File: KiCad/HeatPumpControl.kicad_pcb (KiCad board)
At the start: 2 copper layers, 38.2 x 37.4 mm, 45 parts, among them J1 Conn_01x04_Male, J2 Conn_01x04_Male, J3 Conn_01x04_Male, J4 Conn_01x03_Male, Q1 2N2222A, Q2 Q_PMOS_GDS, U3 XIAO-ESP32-C6-SMD

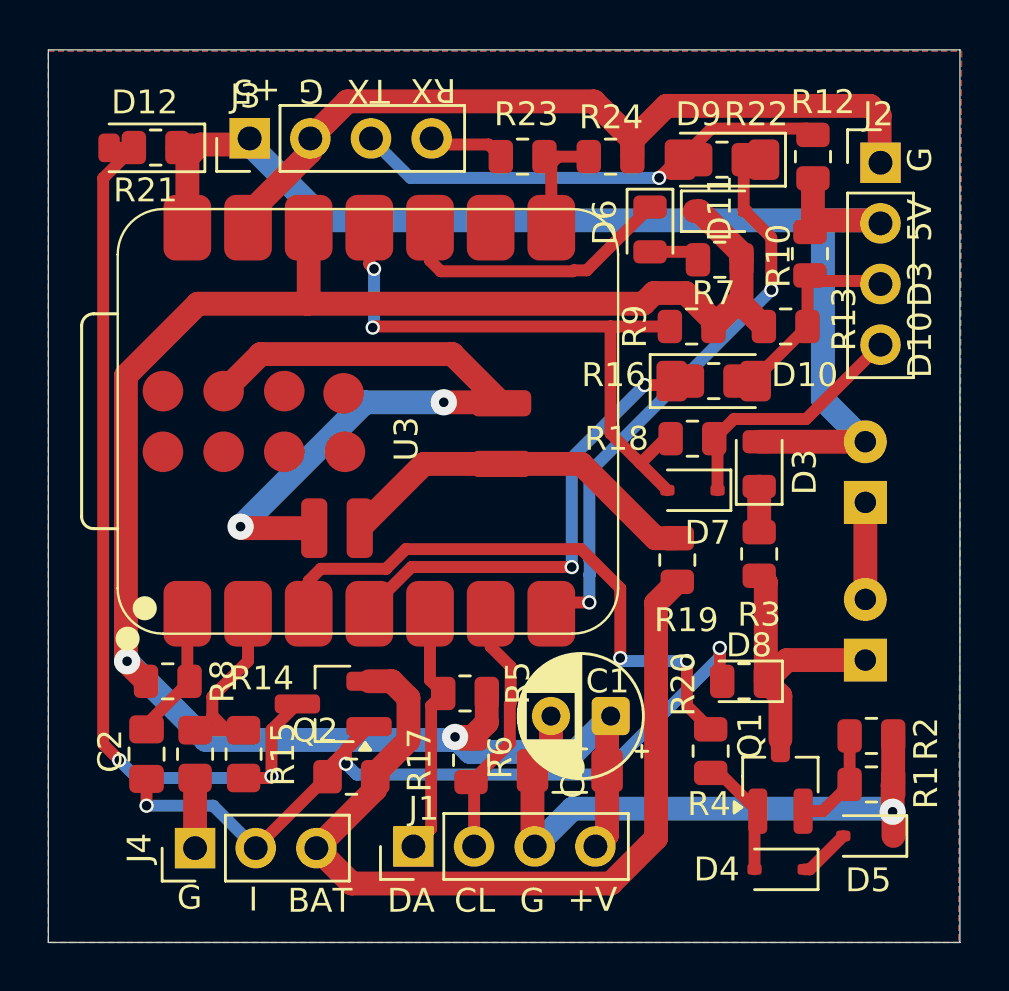
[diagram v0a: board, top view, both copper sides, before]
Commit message: Fill zones updated
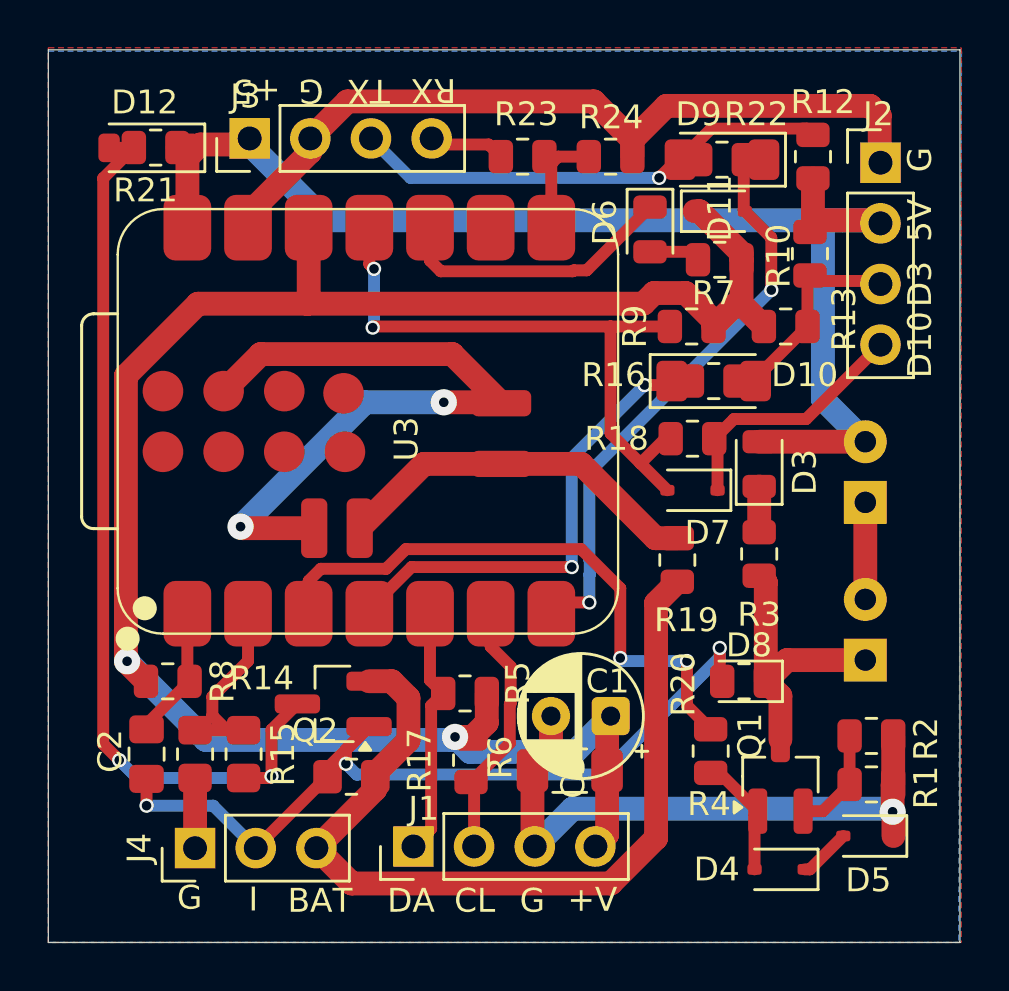
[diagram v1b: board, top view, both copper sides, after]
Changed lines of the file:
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@@
 		(net 1)
 		(net_name "GND")
-		(layers "F.Cu" "B.Cu")
+		(layer "F.Cu")
+		(name "FZoneGnd")
+		(hatch edge 0.508)
+		(priority 2)
+		(connect_pads
+			(clearance 0.508)
+		)
+		(min_thickness 0.254)
+		(filled_areas_thickness no)
+		(fill yes
+			(thermal_gap 0.508)
+			(thermal_bridge_width 0.508)
+		)
+		(polygon
+			(pts
+				(xy 135.89 123.825) (xy 135.89 86.36) (xy 174.117 86.36) (xy 174.117 123.825)
+			)
+		)
+	)
+	(zone
+		(net 1)
+		(net_name "GND")
+		(layer "B.Cu")
+		(name "BZoneGnd")
 		(hatch edge 0.508)
 		(connect_pads
